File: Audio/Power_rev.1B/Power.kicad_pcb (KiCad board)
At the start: 2 copper layers, 96.5 x 101.6 mm, 38 parts, among them P1 CONN_01X02, P2 CONN_01X02, P3 CONN_01X02, P4 CONN_01X02, Q1 NPN(TO-220-BCE), Q2 PNP(TO-220-BCE), Q3 NPN(TO-220-BCE), Q4 PNP(TO-220-BCE)

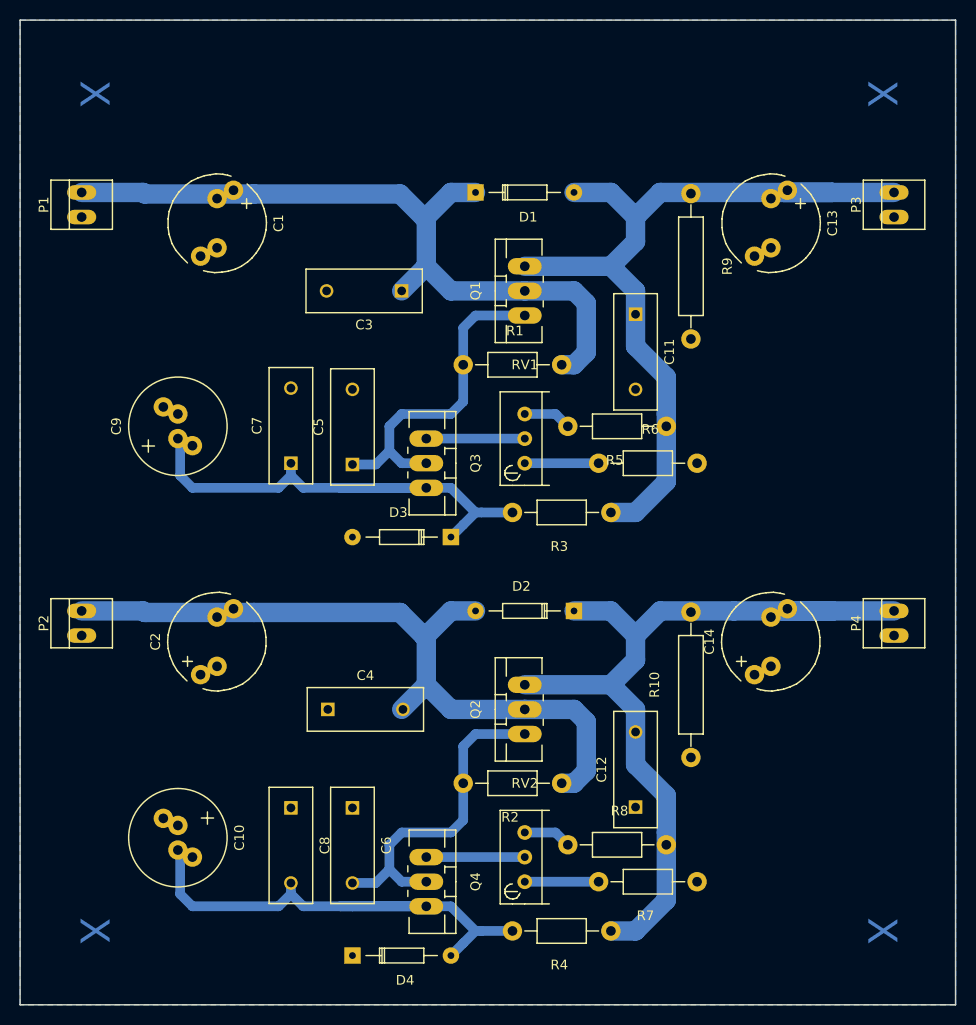
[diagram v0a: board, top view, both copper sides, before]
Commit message: Fix
Fixed for ERC cpmpliance.
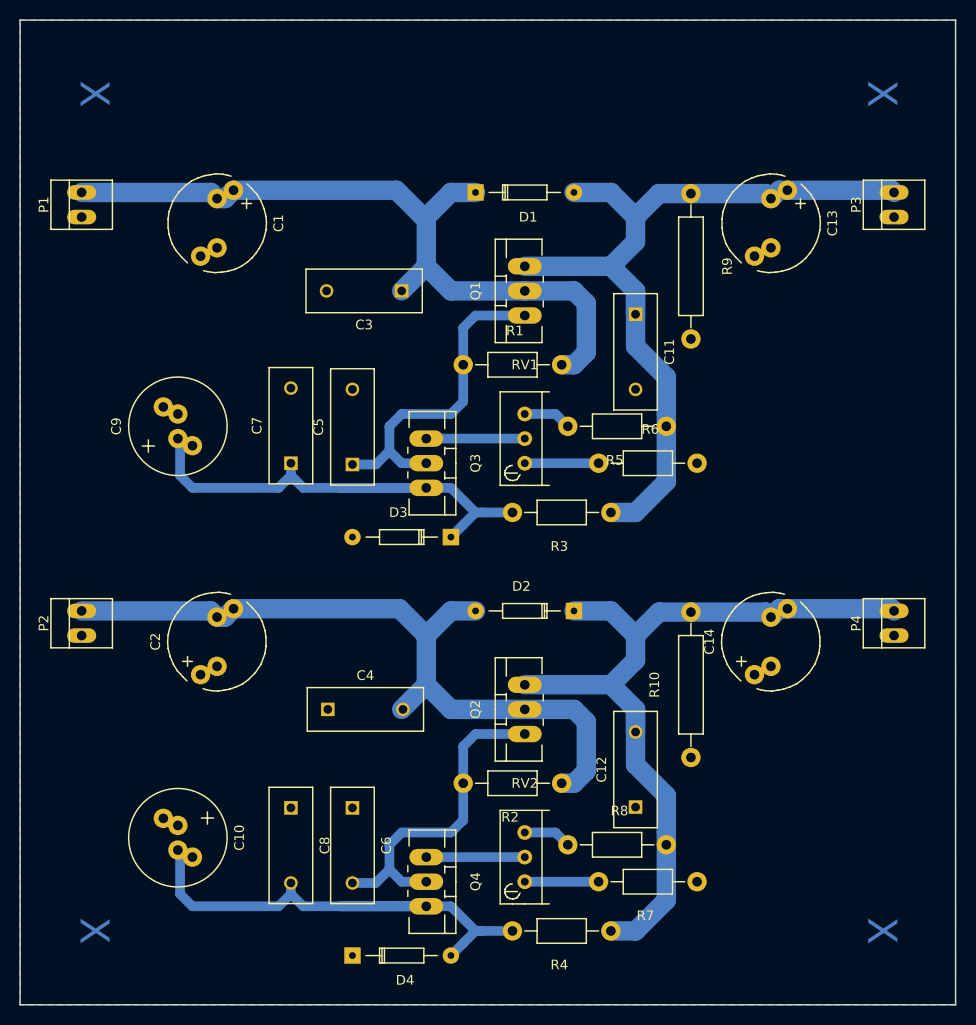
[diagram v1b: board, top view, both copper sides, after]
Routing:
- net VEE: track 91.9 -> 84.7 mm
- net VCC: track 91.9 -> 84.8 mm
- net 63-75V(-): track 77.7 -> 78.4 mm
- net 63-75V(+): track 77.7 -> 78.4 mm
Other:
- net class Default: clearance 0.2 -> 0.6
- net class Large: clearance 0.2 -> 0.6
- rule trace_clearance: 0.2 -> 0.6
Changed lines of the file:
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@@
     (thickness 1.6)
     (drawings 16)
-    (tracks 136)
+    (tracks 144)
     (zones 0)
     (modules 38)
@@
   (setup
     (last_trace_width 1)
-    (trace_clearance 0.2)
+    (trace_clearance 0.6)
     (zone_clearance 0.508)
     (zone_45_only no)
@@
   (net 15 "Net-(R8-Pad1)")
   (net_class Default "This is the default net class."
-    (clearance 0.2)
+    (clearance 0.6)
     (trace_width 1)
     (via_dia 0.6)
@@
   )
   (net_class Large ""
-    (clearance 0.2)
+    (clearance 0.6)
     (trace_width 2)
     (via_dia 0.6)
@@
   (gr_line (start 68.58 22.86) (end 68.58 20.32) (angle 90) (layer Dwgs.User) (width 0.2))
   (gr_line (start 20.32 71.12) (end 116.84 71.12) (angle 90) (layer Dwgs.User) (width 0.2))
+  (segment (start 40.64 38.735) (end 40.005 38.1) (width 2) (layer B.Cu) (net 1))
+  (segment (start 40.005 38.1) (end 26.67 38.1) (width 2) (layer B.Cu) (net 1))
+  (segment (start 42.33926 37.87394) (end 59.14394 37.87394) (width 2) (layer B.Cu) (net 1))
+  (segment (start 59.14394 37.87394) (end 59.53 38.26) (width 2) (layer B.Cu) (net 1))
+  (segment (start 40.64 38.735) (end 41.4782 38.735) (width 2) (layer B.Cu) (net 1))
+  (segment (start 41.4782 38.735) (end 42.33926 37.87394) (width 2) (layer B.Cu) (net 1))
   (segment (start 59.53 38.26) (end 61.91 40.64) (width 2) (layer B.Cu) (net 1))
-  (segment (start 26.67 38.1) (end 33.02 38.1) (width 2) (layer B.Cu) (net 1))
-  (segment (start 33.18 38.26) (end 33.02 38.1) (width 2) (layer B.Cu) (net 1))
-  (segment (start 44.45 38.26) (end 33.18 38.26) (width 2) (layer B.Cu) (net 1))
-  (segment (start 44.45 38.26) (end 59.53 38.26) (width 2) (layer B.Cu) (net 1))
   (segment (start 61.91 40.64) (end 62.23 40.64) (width 2) (layer B.Cu) (net 1))
   (segment (start 59.69 48.26) (end 62.23 45.72) (width 2) (layer B.Cu) (net 1))
@@
   (segment (start 62.23 40.64) (end 62.23 45.72) (width 2) (layer B.Cu) (net 1))
   (segment (start 64.77 48.26) (end 72.39 48.26) (width 2) (layer B.Cu) (net 1))
+  (segment (start 83.82 50.67) (end 83.82 48.26) (width 2) (layer B.Cu) (net 3))
+  (segment (start 89.535 38.22) (end 86.24 38.22) (width 2) (layer B.Cu) (net 3))
+  (segment (start 86.24 38.22) (end 83.82 40.64) (width 2) (layer B.Cu) (net 3))
+  (segment (start 99.48926 37.87394) (end 98.65106 37.87394) (width 2) (layer B.Cu) (net 3))
+  (segment (start 98.65106 37.87394) (end 97.79 38.735) (width 2) (layer B.Cu) (net 3))
+  (segment (start 89.535 38.22) (end 97.275 38.22) (width 2) (layer B.Cu) (net 3))
+  (segment (start 97.275 38.22) (end 97.79 38.735) (width 2) (layer B.Cu) (net 3))
+  (segment (start 99.48926 37.87394) (end 110.26394 37.87394) (width 2) (layer B.Cu) (net 3))
+  (segment (start 110.26394 37.87394) (end 110.49 38.1) (width 2) (layer B.Cu) (net 3))
   (segment (start 86.995 57.15) (end 83.82 53.975) (width 2) (layer B.Cu) (net 3))
   (segment (start 81.28 45.72) (end 83.82 48.26) (width 2) (layer B.Cu) (net 3))
@@
   (segment (start 86.995 60.96) (end 86.995 67.945) (width 2) (layer B.Cu) (net 3))
   (segment (start 83.82 48.26) (end 83.82 53.975) (width 2) (layer B.Cu) (net 3))
-  (segment (start 93.98 38.1) (end 104.14 38.1) (width 2) (layer B.Cu) (net 3))
-  (segment (start 83.82 40.64) (end 86.36 38.1) (width 2) (layer B.Cu) (net 3))
-  (segment (start 86.36 38.1) (end 93.98 38.1) (width 2) (layer B.Cu) (net 3))
-  (segment (start 104.14 38.1) (end 99.06 38.1) (width 2) (layer B.Cu) (net 3))
-  (segment (start 99.06 38.1) (end 104.14 38.1) (width 2) (layer B.Cu) (net 3))
-  (segment (start 110.49 38.1) (end 104.14 38.1) (width 2) (layer B.Cu) (net 3))
   (segment (start 83.82 40.64) (end 83.82 43.18) (width 2) (layer B.Cu) (net 3))
   (segment (start 81.28 38.1) (end 83.82 40.64) (width 2) (layer B.Cu) (net 3))
@@
   (segment (start 77.47 38.1) (end 81.28 38.1) (width 2) (layer B.Cu) (net 3))
   (segment (start 81.28 45.72) (end 72.39 45.72) (width 2) (layer B.Cu) (net 3))
+  (segment (start 40.64 81.915) (end 40.005 81.28) (width 2) (layer B.Cu) (net 4))
+  (segment (start 40.005 81.28) (end 26.67 81.28) (width 2) (layer B.Cu) (net 4))
+  (segment (start 40.64 81.915) (end 41.4782 81.915) (width 2) (layer B.Cu) (net 4))
+  (segment (start 41.4782 81.915) (end 42.33926 81.05394) (width 2) (layer B.Cu) (net 4))
+  (segment (start 42.33926 81.05394) (end 59.46394 81.05394) (width 2) (layer B.Cu) (net 4))
+  (segment (start 59.46394 81.05394) (end 62.23 83.82) (width 2) (layer B.Cu) (net 4))
   (segment (start 64.77 91.44) (end 72.39 91.44) (width 2) (layer B.Cu) (net 4))
   (segment (start 62.23 83.82) (end 62.23 88.9) (width 2) (layer B.Cu) (net 4))
@@
   (segment (start 76.2 99.06) (end 77.47 99.06) (width 2) (layer B.Cu) (net 4))
   (segment (start 59.69 91.44) (end 62.23 88.9) (width 2) (layer B.Cu) (net 4))
-  (segment (start 61.91 83.82) (end 62.23 83.82) (width 2) (layer B.Cu) (net 4))
-  (segment (start 44.45 81.44) (end 59.53 81.44) (width 2) (layer B.Cu) (net 4))
-  (segment (start 44.45 81.44) (end 33.18 81.44) (width 2) (layer B.Cu) (net 4))
-  (segment (start 33.18 81.44) (end 33.02 81.28) (width 2) (layer B.Cu) (net 4))
-  (segment (start 26.67 81.28) (end 33.02 81.28) (width 2) (layer B.Cu) (net 4))
-  (segment (start 59.53 81.44) (end 61.91 83.82) (width 2) (layer B.Cu) (net 4))
   (segment (start 62.23 111.76) (end 53.34 111.76) (width 1) (layer B.Cu) (net 5))
   (segment (start 57.15 111.76) (end 62.23 111.76) (width 1) (layer B.Cu) (net 5))
@@
   (segment (start 64.77 116.84) (end 66.04 115.57) (width 1) (layer B.Cu) (net 5))
   (segment (start 66.04 115.57) (end 67.31 114.3) (width 1) (layer B.Cu) (net 5))
+  (segment (start 83.82 93.77) (end 83.82 91.44) (width 2) (layer B.Cu) (net 6))
+  (segment (start 89.535 81.4) (end 86.24 81.4) (width 2) (layer B.Cu) (net 6))
+  (segment (start 86.24 81.4) (end 83.82 83.82) (width 2) (layer B.Cu) (net 6))
+  (segment (start 99.48926 81.05394) (end 98.65106 81.05394) (width 2) (layer B.Cu) (net 6))
+  (segment (start 98.65106 81.05394) (end 97.79 81.915) (width 2) (layer B.Cu) (net 6))
+  (segment (start 89.535 81.4) (end 97.275 81.4) (width 2) (layer B.Cu) (net 6))
+  (segment (start 97.275 81.4) (end 97.79 81.915) (width 2) (layer B.Cu) (net 6))
+  (segment (start 99.48926 81.05394) (end 110.26394 81.05394) (width 2) (layer B.Cu) (net 6))
+  (segment (start 110.26394 81.05394) (end 110.49 81.28) (width 2) (layer B.Cu) (net 6))
   (segment (start 81.28 88.9) (end 72.39 88.9) (width 2) (layer B.Cu) (net 6))
   (segment (start 77.47 81.28) (end 81.28 81.28) (width 2) (layer B.Cu) (net 6))
@@
   (segment (start 81.28 81.28) (end 83.82 83.82) (width 2) (layer B.Cu) (net 6))
   (segment (start 83.82 83.82) (end 83.82 86.36) (width 2) (layer B.Cu) (net 6))
-  (segment (start 110.49 81.28) (end 104.14 81.28) (width 2) (layer B.Cu) (net 6))
-  (segment (start 99.06 81.28) (end 104.14 81.28) (width 2) (layer B.Cu) (net 6))
-  (segment (start 104.14 81.28) (end 99.06 81.28) (width 2) (layer B.Cu) (net 6))
-  (segment (start 86.36 81.28) (end 93.98 81.28) (width 2) (layer B.Cu) (net 6))
-  (segment (start 83.82 83.82) (end 86.36 81.28) (width 2) (layer B.Cu) (net 6))
-  (segment (start 93.98 81.28) (end 104.14 81.28) (width 2) (layer B.Cu) (net 6))
   (segment (start 83.82 91.44) (end 83.82 97.155) (width 2) (layer B.Cu) (net 6))
   (segment (start 86.995 104.14) (end 86.995 111.125) (width 2) (layer B.Cu) (net 6))

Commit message: further tweaking(1)
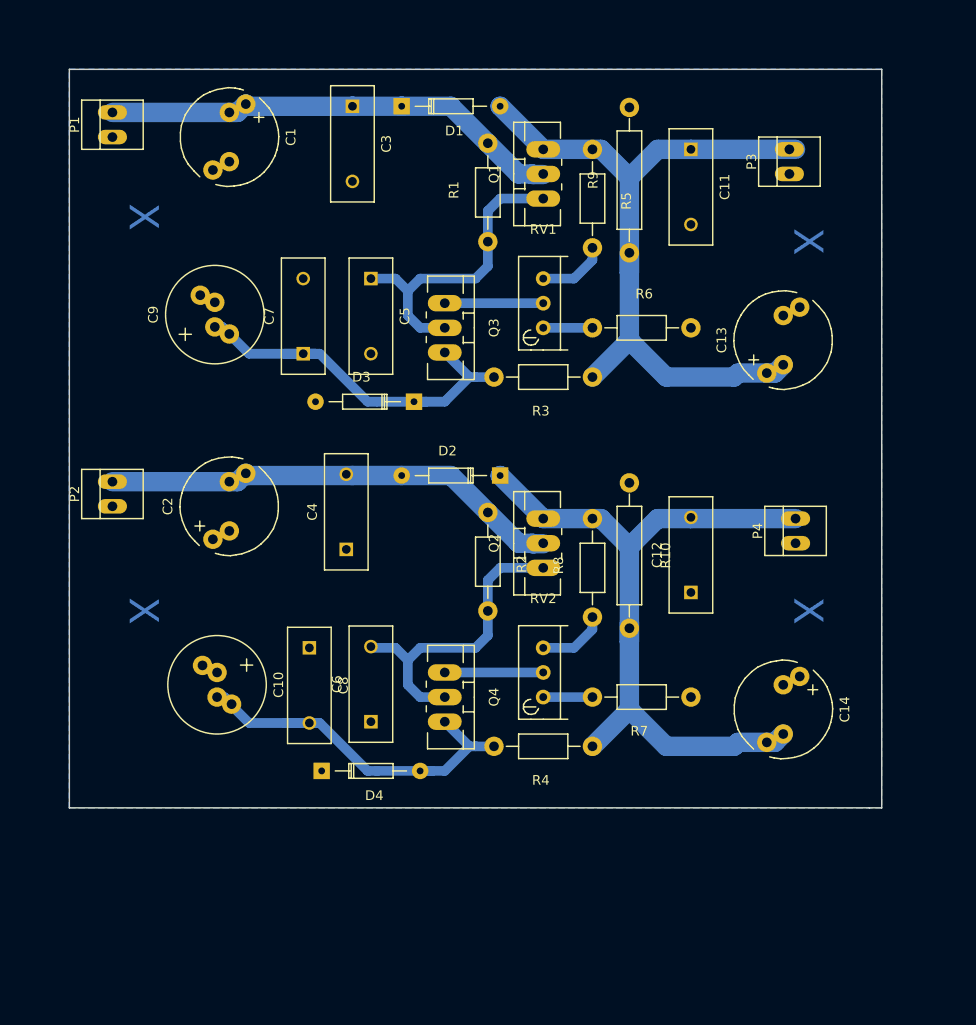
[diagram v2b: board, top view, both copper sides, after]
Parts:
- moved R8 28.7 mm to (79.4, 76.8), turned to 90 degrees
- moved R5 23.6 mm to (79.4, 38.7), turned to 270 degrees
- moved R2 23.0 mm to (68.6, 76.2), turned to 270 degrees
- moved C12 22.9 mm to (89.5, 79.4)
- moved C3 19.7 mm to (54.6, 29.2), turned to 270 degrees
- moved D4 19.3 mm to (51.4, 97.8)
- moved C5 19.3 mm to (56.5, 47.0), turned to 270 degrees
- moved Q4 19.1 mm to (64.1, 90.2)
- moved R4 19.1 mm to (74.3, 95.2)
- moved RV2 19.1 mm to (74.3, 90.2)
- moved R7 19.1 mm to (84.5, 90.2)
- moved R1 18.0 mm to (68.6, 38.1), turned to 90 degrees
- moved C11 17.9 mm to (89.5, 33.7)
- moved Q2 17.3 mm to (74.3, 74.3)
- moved C4 16.6 mm to (54.0, 74.9), turned to 90 degrees
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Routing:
- net 63-75V(-): track 78.4 -> 47.8 mm
- net 63-75V(+): track 78.4 -> 47.8 mm
- net Net-(C10-Pad2): track 54.5 -> 42.4 mm
- net Net-(C7-Pad1): track 54.5 -> 42.4 mm
- net VCC: track 84.8 -> 77.0 mm
- net VEE: track 84.7 -> 77.0 mm
- net Net-(R7-Pad2): track 7.62 -> 5.08 mm
- net Net-(R6-Pad1): track 7.62 -> 5.08 mm
- net Net-(R5-Pad2): track 4.97 -> 7.14 mm
- net Net-(R8-Pad1): track 4.97 -> 7.14 mm
- net Net-(C5-Pad1): track 34.4 -> 32.5 mm
- net Net-(C6-Pad2): track 34.4 -> 32.5 mm
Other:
- board size 96.5 x 101.6 mm -> 83.8 x 76.2 mm
